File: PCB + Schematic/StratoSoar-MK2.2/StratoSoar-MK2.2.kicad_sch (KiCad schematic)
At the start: 114 parts, among them J1 BME280, J10 Rudder, J11 Elevator, J12 Parachute, J13 GY-91, J14 VOUT, J15 VIN, J2 FTDI, J3 AT_ISP, J4 Signal, J5 USB-C, J6 SWD, J7 Power, J8 Button, J9 VIN, Q1 2N3906, Q2 2N3906, Q3 2N3906, Q4 DMN1019USN-13, Q5 DMN1019USN-13, Q6 DMN1019USN-13, SW1 AT_RESET, SW2 EEPROM, SW3 AAA, SW4 PWR_SW, SW5 RESET, U1 MAX-M10S, U2 MPU-9250, U3 ATmega328P-A, U4 AT24C512C-SSHD-T, U5 ATXK-H11-E-32.768, U6 ATSAMD21G18A-A, U7 MCP1700x-330xxTT, Y1 8MHz, Y2 32.768kHz

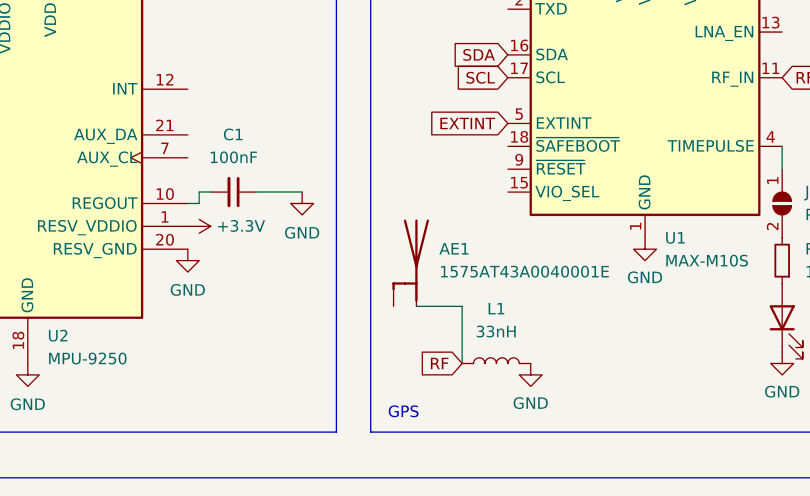
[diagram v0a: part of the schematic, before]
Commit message: Finish new PCB
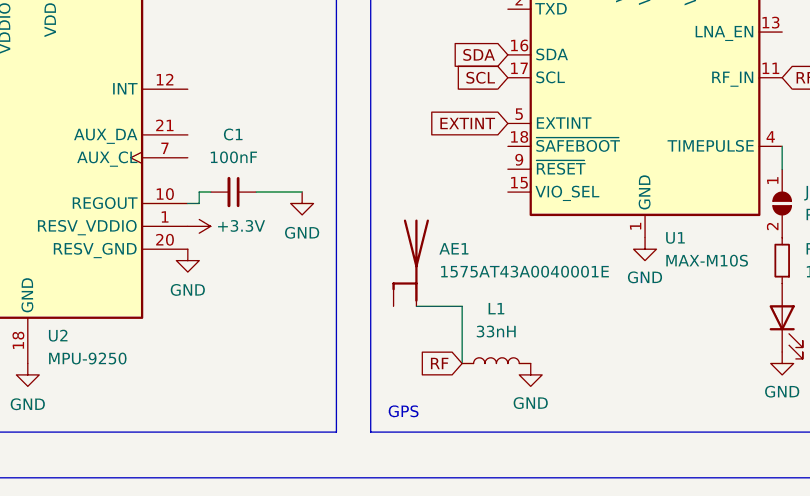
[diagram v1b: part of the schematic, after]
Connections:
- net RF: now also AE1.1 (FEED); no longer AE1.2 (RF)
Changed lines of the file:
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@@
 			)
 		)
-		(property "Description" ""
+		(property "Description" "Ceramic chip antenna with pin for PCB trace"
 			(at 331.47 382.27 0)
 			(effects
